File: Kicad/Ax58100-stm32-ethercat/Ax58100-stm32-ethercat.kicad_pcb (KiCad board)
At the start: 2 copper layers, 95.3 x 89.4 mm, 166 parts, among them J1 Out_opt, J10 5V Power IN, J11 Step1, J12 Serial usart1, J13 Step2, J15 In1-4, J16 24V Field, J17 In5-8, J19 Step3, J2 Output1-2, J20 Step4, J21 THCAD, J3 In_opt1, J4 Output3-4, J5 In_opt2, J6 DAC, J7 Encoder, J9 STLINK, SW1 SW PB, U1 AMS1117-1.2, U10 TXB0104PW, U11 MAX3485CSA/ESA, U2 AX58100, U3 24LC32A, U4 STM32F407VGT6, U5 AMS1117-3.3, U6 TLP292-4, U7 TLP291-4, U8 TLP292-4, U9 TXB0104PW, Y1 NXK25.000AE12F-KAB6-12, Y2 8 MHz

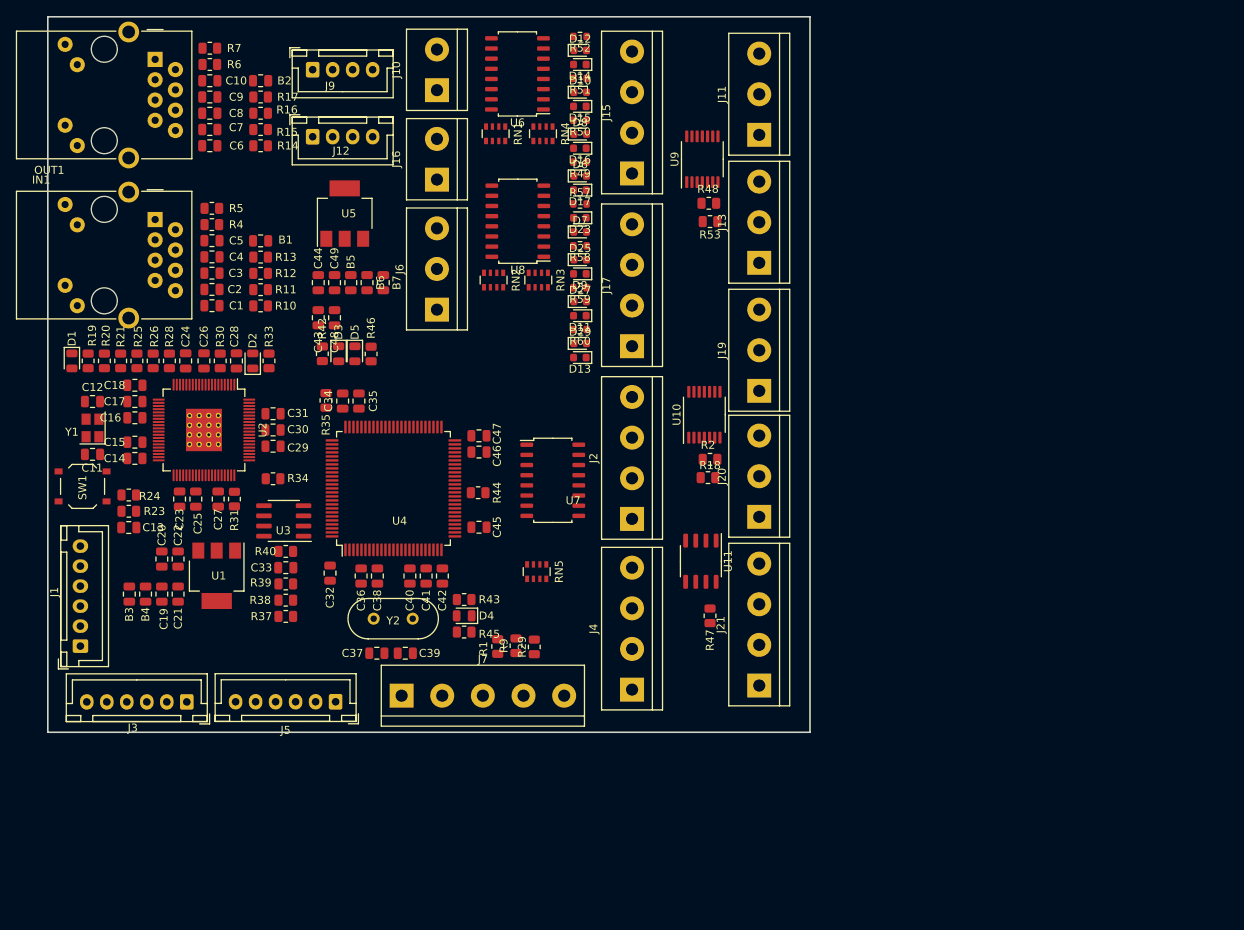
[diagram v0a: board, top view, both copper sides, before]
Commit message: wip
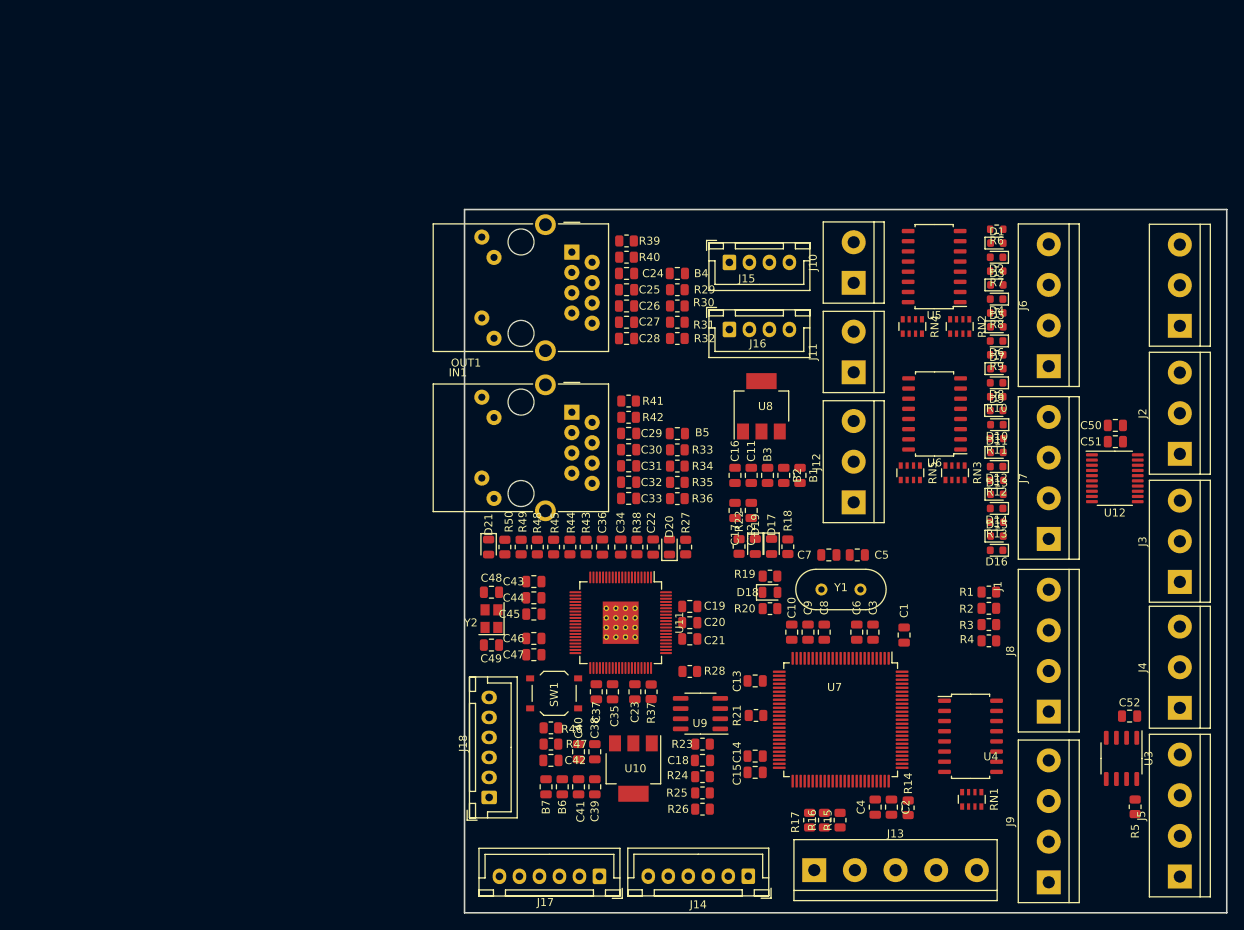
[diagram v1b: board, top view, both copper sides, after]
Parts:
- removed the U10 at (116.1, 74.6)
- removed the U9 at (115.8, 42.7)
- added C50: 0.1uF, Capacitor_SMD:C_0805_2012Metric, F.Cu at (167.5, 75.9)
- added C51: 0.1uF, Capacitor_SMD:C_0805_2012Metric, F.Cu at (167.5, 78.0)
- added C52: 0.1uF, Capacitor_SMD:C_0805_2012Metric, F.Cu at (169.2, 112.3)
- added U12: TXS0108EPW, Package_SO:TSSOP-20_4.4x6.5mm_P0.65mm, F.Cu at (167.4, 82.5)
- U4: renamed from U7; value TLP291-4 -> TLP292-4
- moved R14 88.8 mm to (141.6, 123.7), turned to -90 degrees
- moved C2 85.3 mm to (139.5, 123.7), turned to -90 degrees
- moved C4 82.1 mm to (137.4, 123.7), turned to 90 degrees
- moved C1 72.2 mm to (141.0, 102.1), turned to 90 degrees
- moved SW1 64.4 mm to (97.3, 109.4)
- moved C3 64.4 mm to (137.2, 101.8), turned to 90 degrees
- moved U7 62.9 mm to (133.1, 112.7), turned to -90 degrees
- moved RN1 61.4 mm to (149.5, 122.7)
- moved C5 61.3 mm to (135.2, 92.1), turned to 0 degrees
- moved U4 61.2 mm to (149.4, 114.8)
- moved C6 60.3 mm to (135.1, 101.8), turned to 90 degrees
- moved C42 60.3 mm to (96.9, 117.8)
- moved R47 60.3 mm to (96.9, 115.8)
- moved R46 60.3 mm to (96.9, 113.8)
- moved R1 59.9 mm to (151.6, 96.8)
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- renumbered B7 to B1, B6 to B2, B5 to B3, B2 to B4, B1 to B5, B4 to B6, B3 to B7, C32 to C1, C42 to C10, C49 to C11, C48 to C12, C45 to C13, C46 to C14, C47 to C15, C44 to C16, C43 to C17, C33 to C18, C31 to C19, C34 to C2, C30 to C20, C29 to C21, C28 to C22, C27 to C23, C10 to C24, C9 to C25, C8 to C26, C7 to C27, C6 to C28, C5 to C29, C36 to C3, C4 to C30, C3 to C31, C2 to C32, C1 to C33, C26 to C34, C25 to C35, C24 to C36, C23 to C37, C22 to C38, C21 to C39, C35 to C4, C20 to C40, C19 to C41, C13 to C42, C18 to C43, C17 to C44, C16 to C45, C15 to C46, C14 to C47, C12 to C48, C11 to C49, C37 to C5, C38 to C6, C39 to C7, C40 to C8, C41 to C9, D12 to D1, D7 to D10, D25 to D11, D9 to D12, D27 to D13, D11 to D14, D29 to D15, D13 to D16, D5 to D17, D4 to D18, D3 to D19, D14 to D2, D2 to D20, D1 to D21, D10 to D3, D15 to D4, D8 to D5, D16 to D6, D6 to D7, D17 to D8, D23 to D9, J11 to J1, J16 to J11, J6 to J12, J7 to J13, J5 to J14, J9 to J15, J12 to J16, J3 to J17, J1 to J18, J13 to J2, J19 to J3, J20 to J4, J21 to J5, J15 to J6, J17 to J7, J2 to J8, J4 to J9, R48 to R1, R57 to R10, R58 to R11, R59 to R12, R60 to R13, R35 to R14, R29 to R15, R9 to R16, R1 to R17, R46 to R18, R45 to R19, R53 to R2, R43 to R20, R44 to R21, R42 to R22, R40 to R23, R39 to R24, R38 to R25, R37 to R26, R33 to R27, R34 to R28, R17 to R29, R2 to R3, R16 to R30, R15 to R31, R14 to R32, R13 to R33, R12 to R34, R11 to R35, R10 to R36, R31 to R37, R30 to R38, R7 to R39, R18 to R4, R6 to R40, R5 to R41, R4 to R42, R28 to R43, R26 to R44, R25 to R45, R24 to R46, R23 to R47, R21 to R48, R20 to R49, R47 to R5, R19 to R50, R52 to R6, R51 to R7, R50 to R8, R49 to R9, RN5 to RN1, RN4 to RN2, RN1 to RN4, RN2 to RN5, U1 to U10, U2 to U11, U11 to U3, U6 to U5, U8 to U6, U4 to U7, U5 to U8, U3 to U9, Y2 to Y1, Y1 to Y2
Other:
- board size 95.3 x 89.4 mm -> 95.3 x 87.9 mm
